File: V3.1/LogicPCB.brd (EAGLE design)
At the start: 171.9 x 151.6 mm, 65 parts, among them CON1 CUBE_ORANGE_, CON10 PINHEAD_1X02-2.54, CON11 CON-4P-JST-XA, CON12 PINHEAD_1X06-2.54, CON13 CON-6P-JST-XA, CON14 PINHEAD_1X04-2.54, CON15 CON-4P-JST-XA, CON17 CON-4P-JST-XA, CON18 CON-6P-JST-XA, CON19 USB-TYPE-C-VERT-PROD, CON2 CON-4P-JST-XA, CON20 PINHEAD_1X06-2.54, CON21 CON-4P-JST-XA, CON22 CON-4P-JST-XA, CON23 CON-4P-JST-XA, CON24 CON-4P-JST-XA, CON25 CON-4P-JST-XA, CON26 CON-4P-JST-XA, CON27 CON-4P-JST-XA, CON28 CON-4P-JST-XA, CON29 CON-4P-JST-XA, CON3 RJ45-NO_SHIELD-5556416-1, CON30 CON-4P-JST-XA, CON32 CON-4P-JST-XA, CON35 CON-12P-JST-XA, CON4 CON-2P-JST-XA, CON5 CON-6P-JST-XA, CON6 CON-4P-JST-XA, CON7 PINHEAD_1X06-2.54, CON9 PINHEAD_1X12-2.54, IC5 AOZ1280, M1 05G_ETHERNET_SWITCH, Q1 IRLML0030, T1 H1102NL, T2 H1102NL, T3 H1102NL, T4 H1102NL

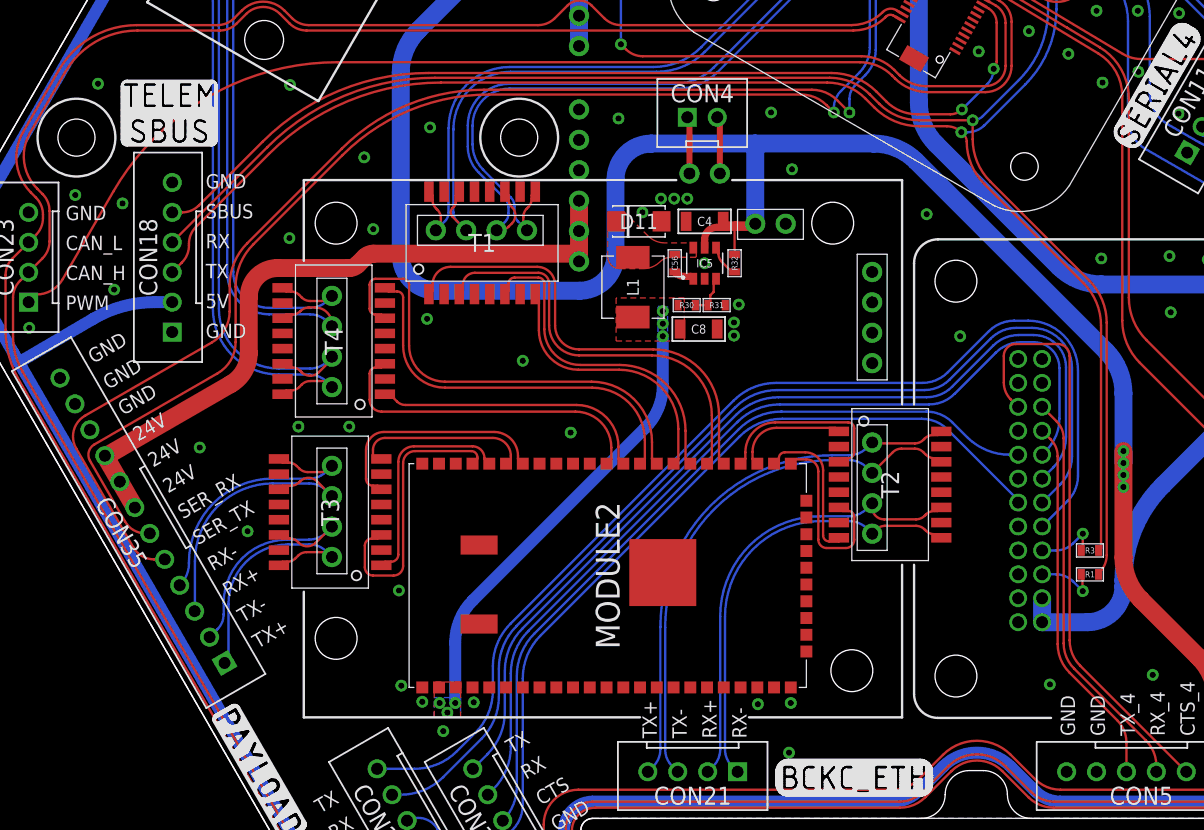
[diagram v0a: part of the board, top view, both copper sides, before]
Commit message: uarts
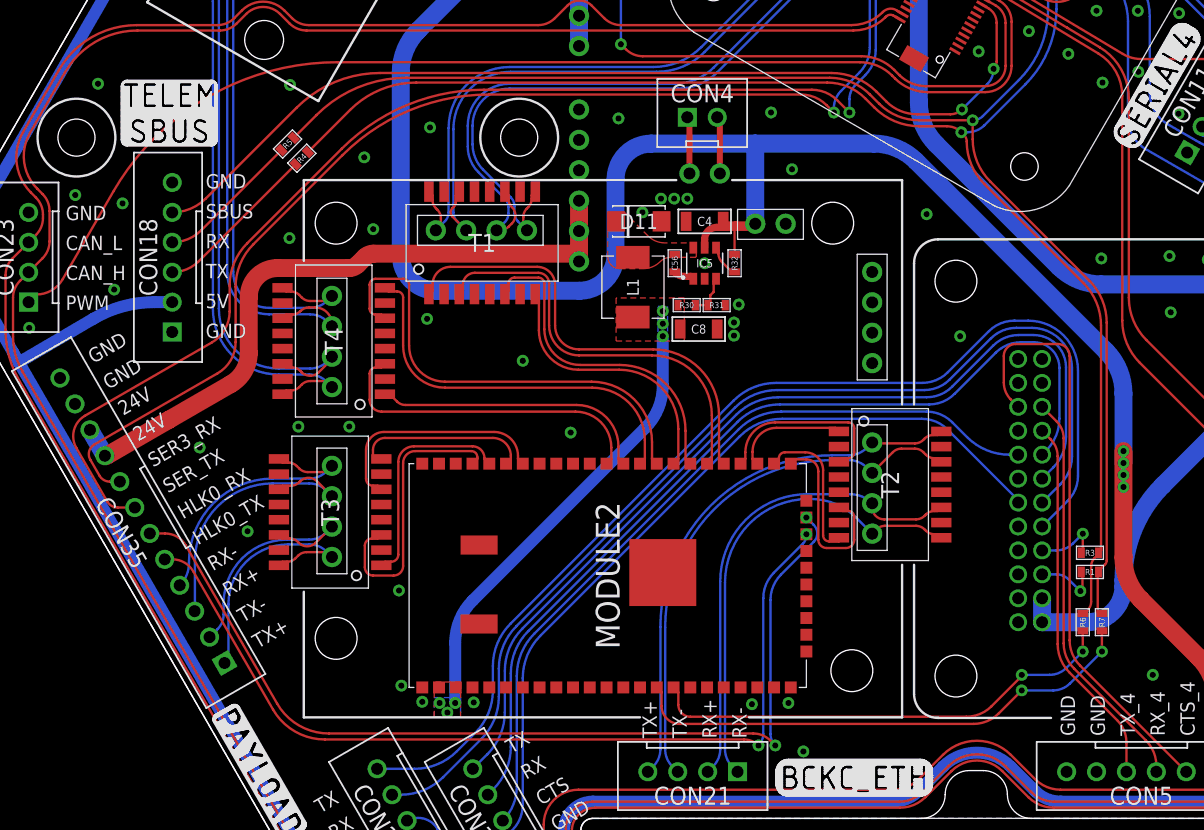
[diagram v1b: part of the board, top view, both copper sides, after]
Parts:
- added R4, R5: (no value), rc:R0603
- added R6, R7: 000, rc:R0603
- moved R1 0.20 mm to (8.70, -26.3)
- moved R3 0.20 mm to (8.70, -24.7)
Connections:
- new net N$10: CON18.4, R5.1
- new net N$9: CON18.3, R4.1
- net GND: no longer CON35.10
- net HLK_RX0: now also CON35.6
- net HLK_RX1: now also R6.1
- net HLK_TX0: now also CON35.5
- net HLK_TX1: now also R7.1
- net SERIAL1_RX: now also R5.2, R7.2; no longer CON18.4
- net SERIAL1_TX: now also R4.2, R6.2; no longer CON18.3
- net SERIAL3_RX: now also CON35.8; no longer CON35.6
- net SERIAL3_TX: now also CON35.7; no longer CON35.5
- net VDD_24V: now also CON35.10; no longer CON35.7, CON35.8
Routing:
- net HLK_RX0: track 0.00 -> 81.8 mm, vias 0 -> 2
- net HLK_TX0: track 0.00 -> 76.3 mm, vias 0 -> 2
- net HLK_TX1: track 0.00 -> 43.1 mm, vias 0 -> 2
- net HLK_RX1: track 0.00 -> 39.6 mm, vias 0 -> 2
- net N$9: track 0.00 -> 13.9 mm
- net N$10: track 0.00 -> 12.1 mm
- net SERIAL1_TX: track 133.7 -> 124.0 mm
- net SERIAL1_RX: track 132.5 -> 123.1 mm
- net SERIAL3_RX: track 121.4 -> 116.5 mm
- net SERIAL3_TX: track 123.7 -> 118.8 mm
- net ETH1_RX-: track 35.4 -> 38.4 mm
- net VDD_24V: track 59.0 -> 56.5 mm
- net ETH1_RX+: track 36.6 -> 38.9 mm
- net GND: vias 114 -> 112
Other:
- board text added: "HLK0_RX"
- board text added: "HLK0_TX"
- board text added: "SER3_RX"
- board text removed: "SER_RX"
